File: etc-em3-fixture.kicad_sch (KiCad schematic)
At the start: 0 parts

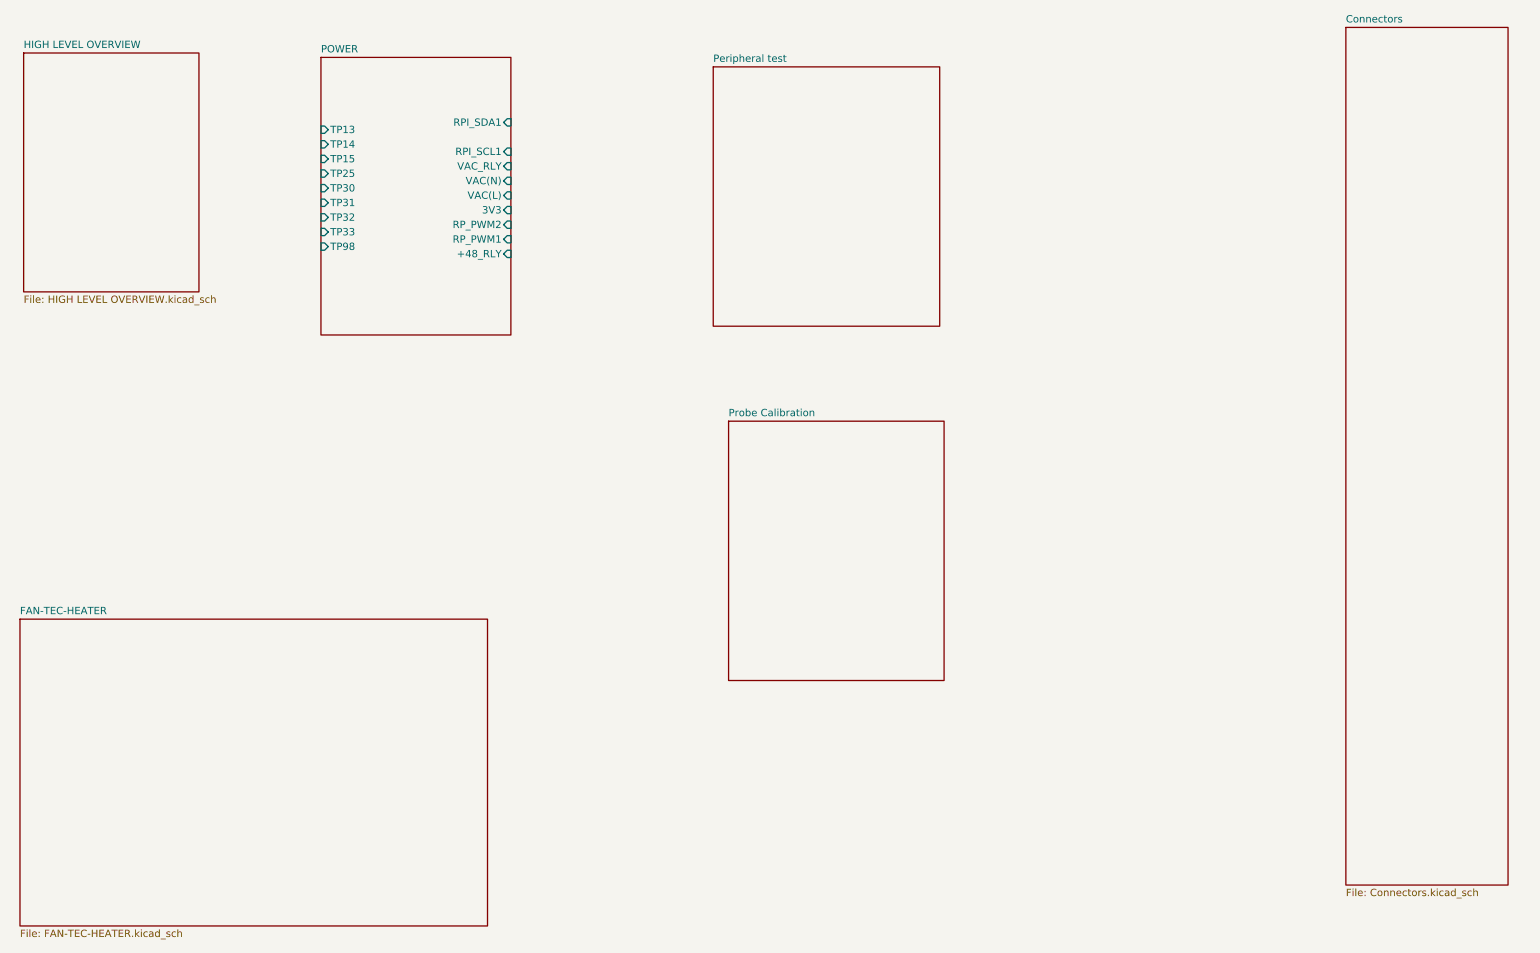
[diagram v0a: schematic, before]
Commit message: latest rev
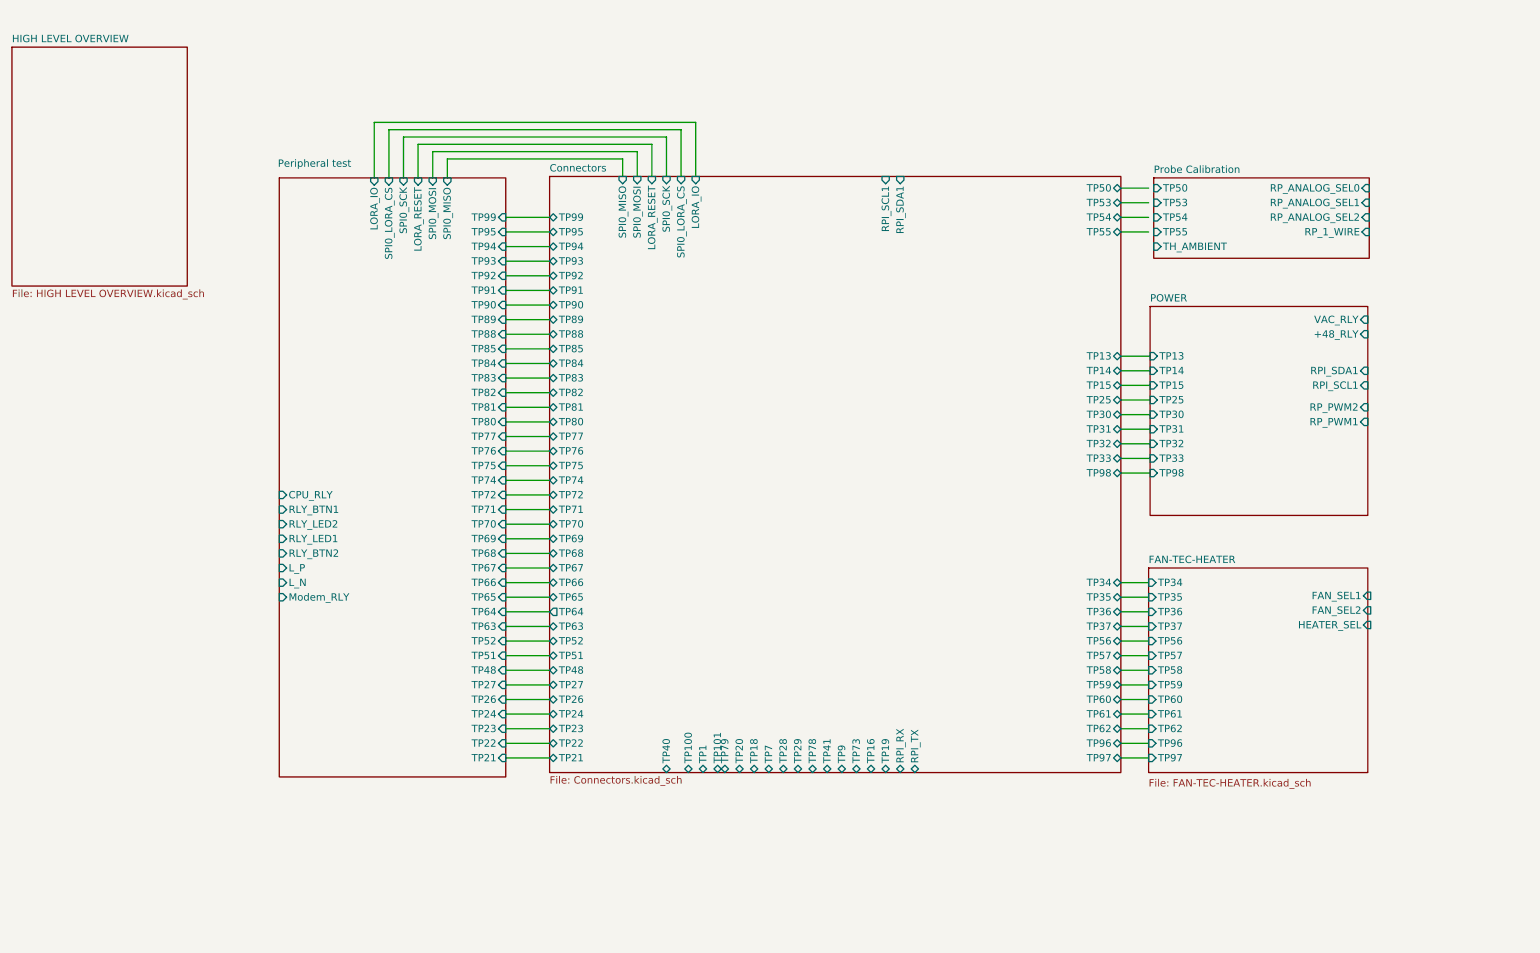
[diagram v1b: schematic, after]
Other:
- sheet Connectors ports: added LORA_IO, LORA_RESET, RPI_RX, RPI_SCL1, RPI_SDA1, RPI_TX, SPI0_LORA_CS, SPI0_MISO, SPI0_MOSI, SPI0_SCK, TP1, TP100, TP101, TP13, TP14, TP15, TP16, TP18, TP19, TP20, TP21, TP22, TP23, TP24, TP25, TP26, TP27, TP28, TP29, TP30, TP31, TP32, TP33, TP34, TP35, TP36, TP37, TP40, TP41, TP48, TP50, TP51, TP52, TP53, TP54, TP55, TP56, TP57, TP58, TP59, TP60, TP61, TP62, TP63, TP64, TP65, TP66, TP67, TP68, TP69, TP7, TP70, TP71, TP72, TP73, TP74, TP75, TP76, TP77, TP78, TP79, TP80, TP81, TP82, TP83, TP84, TP85, TP88, TP89, TP9, TP90, TP91, TP92, TP93, TP94, TP95, TP96, TP97, TP98, TP99; removed none
- sheet FAN-TEC-HEATER ports: added FAN_SEL1, FAN_SEL2, HEATER_SEL, TP34, TP35, TP36, TP37, TP56, TP57, TP58, TP59, TP60, TP61, TP62, TP96, TP97; removed none
- sheet POWER ports: added none; removed 3V3, VAC(L), VAC(N)
- sheet Peripheral test ports: added CPU_RLY, LORA_IO, LORA_RESET, L_N, L_P, Modem_RLY, RLY_BTN1, RLY_BTN2, RLY_LED1, RLY_LED2, SPI0_LORA_CS, SPI0_MISO, SPI0_MOSI, SPI0_SCK, TP21, TP22, TP23, TP24, TP26, TP27, TP48, TP51, TP52, TP63, TP64, TP65, TP66, TP67, TP68, TP69, TP70, TP71, TP72, TP74, TP75, TP76, TP77, TP80, TP81, TP82, TP83, TP84, TP85, TP88, TP89, TP90, TP91, TP92, TP93, TP94, TP95, TP99; removed none
- sheet Probe Calibration ports: added RP_1_WIRE, RP_ANALOG_SEL0, RP_ANALOG_SEL1, RP_ANALOG_SEL2, TH_AMBIENT, TP50, TP53, TP54, TP55; removed none

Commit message: V0.1 for review
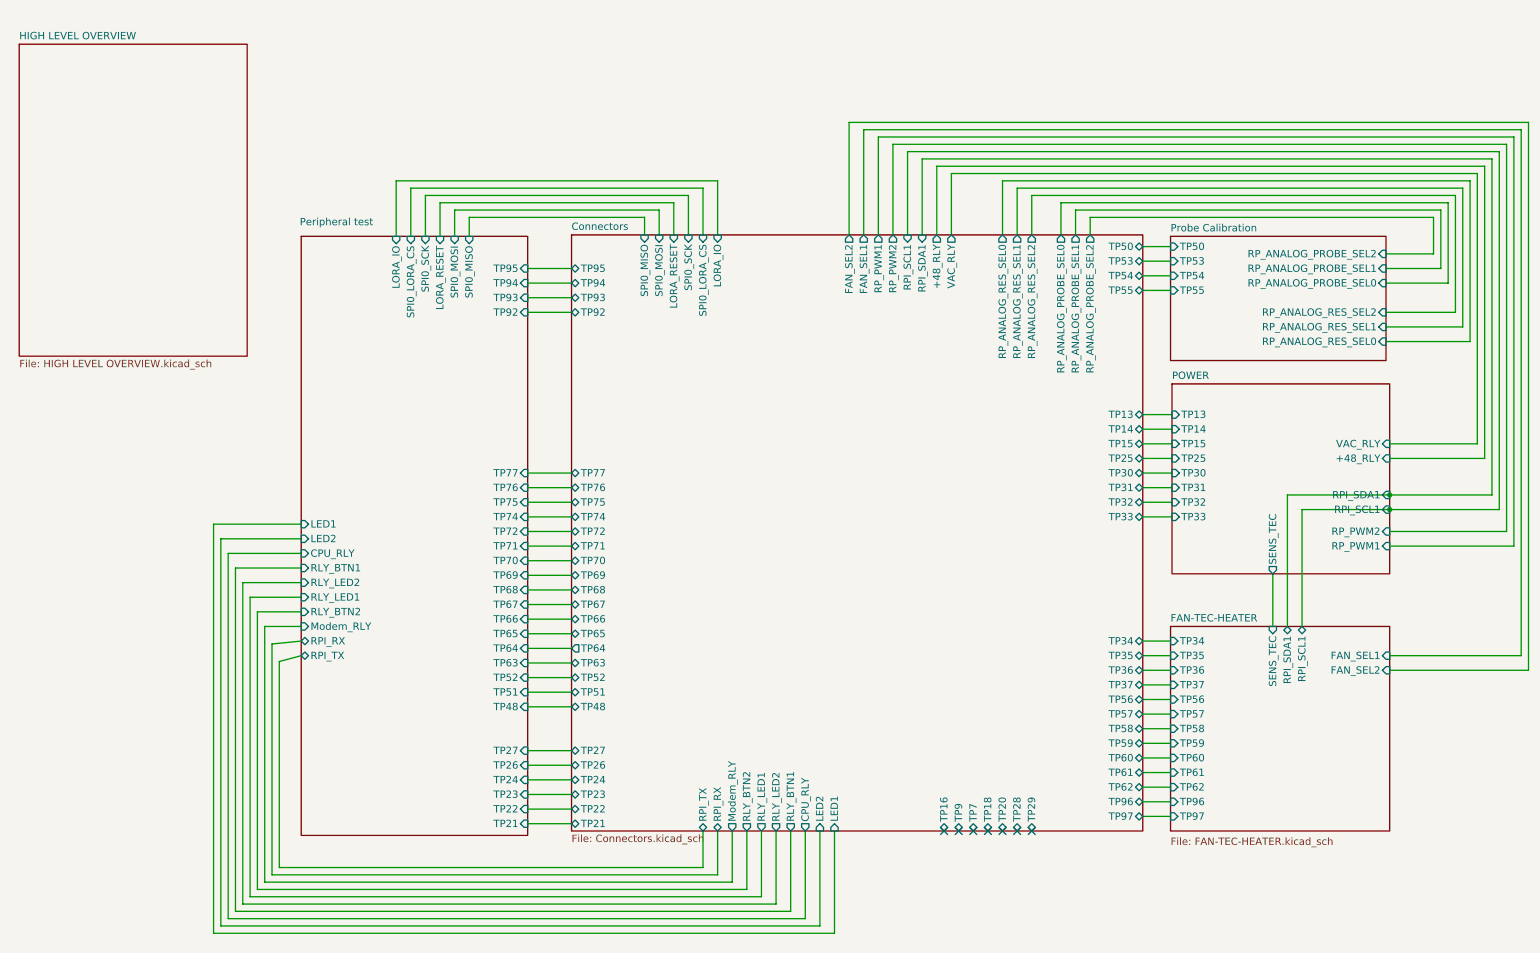
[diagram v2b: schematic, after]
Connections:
- no-connect marks 0 -> 7
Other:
- sheet Connectors ports: added +48_RLY, CPU_RLY, FAN_SEL1, FAN_SEL2, LED1, LED2, Modem_RLY, RLY_BTN1, RLY_BTN2, RLY_LED1, RLY_LED2, RP_ANALOG_PROBE_SEL0, RP_ANALOG_PROBE_SEL1, RP_ANALOG_PROBE_SEL2, RP_ANALOG_RES_SEL0, RP_ANALOG_RES_SEL1, RP_ANALOG_RES_SEL2, RP_PWM1, RP_PWM2, VAC_RLY; removed TP1, TP100, TP101, TP19, TP40, TP41, TP73, TP78, TP79, TP80, TP81, TP82, TP83, TP84, TP85, TP88, TP89, TP90, TP91, TP98, TP99
- sheet FAN-TEC-HEATER ports: added RPI_SCL1, RPI_SDA1, SENS_TEC; removed HEATER_SEL
- sheet POWER ports: added SENS_TEC; removed TP98
- sheet Peripheral test: file Page3.kicad_sch -> Peripheral test.kicad_sch
- sheet Peripheral test ports: added LED1, LED2, RPI_RX, RPI_TX; removed L_N, L_P, TP80, TP81, TP82, TP83, TP84, TP85, TP88, TP89, TP90, TP91, TP99
- sheet Probe Calibration ports: added RP_ANALOG_PROBE_SEL0, RP_ANALOG_PROBE_SEL1, RP_ANALOG_PROBE_SEL2, RP_ANALOG_RES_SEL0, RP_ANALOG_RES_SEL1, RP_ANALOG_RES_SEL2; removed RP_1_WIRE, RP_ANALOG_SEL0, RP_ANALOG_SEL1, RP_ANALOG_SEL2, TH_AMBIENT
